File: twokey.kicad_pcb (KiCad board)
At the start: 2 copper layers, 52.1 x 40 mm, 12 parts, among them J1 12401610E4#2A, SW1 SW_SPST, SW2 SW_SPST, U1 ATSAMD21E18A-A, U2 MCP1700-3302E_SOT23

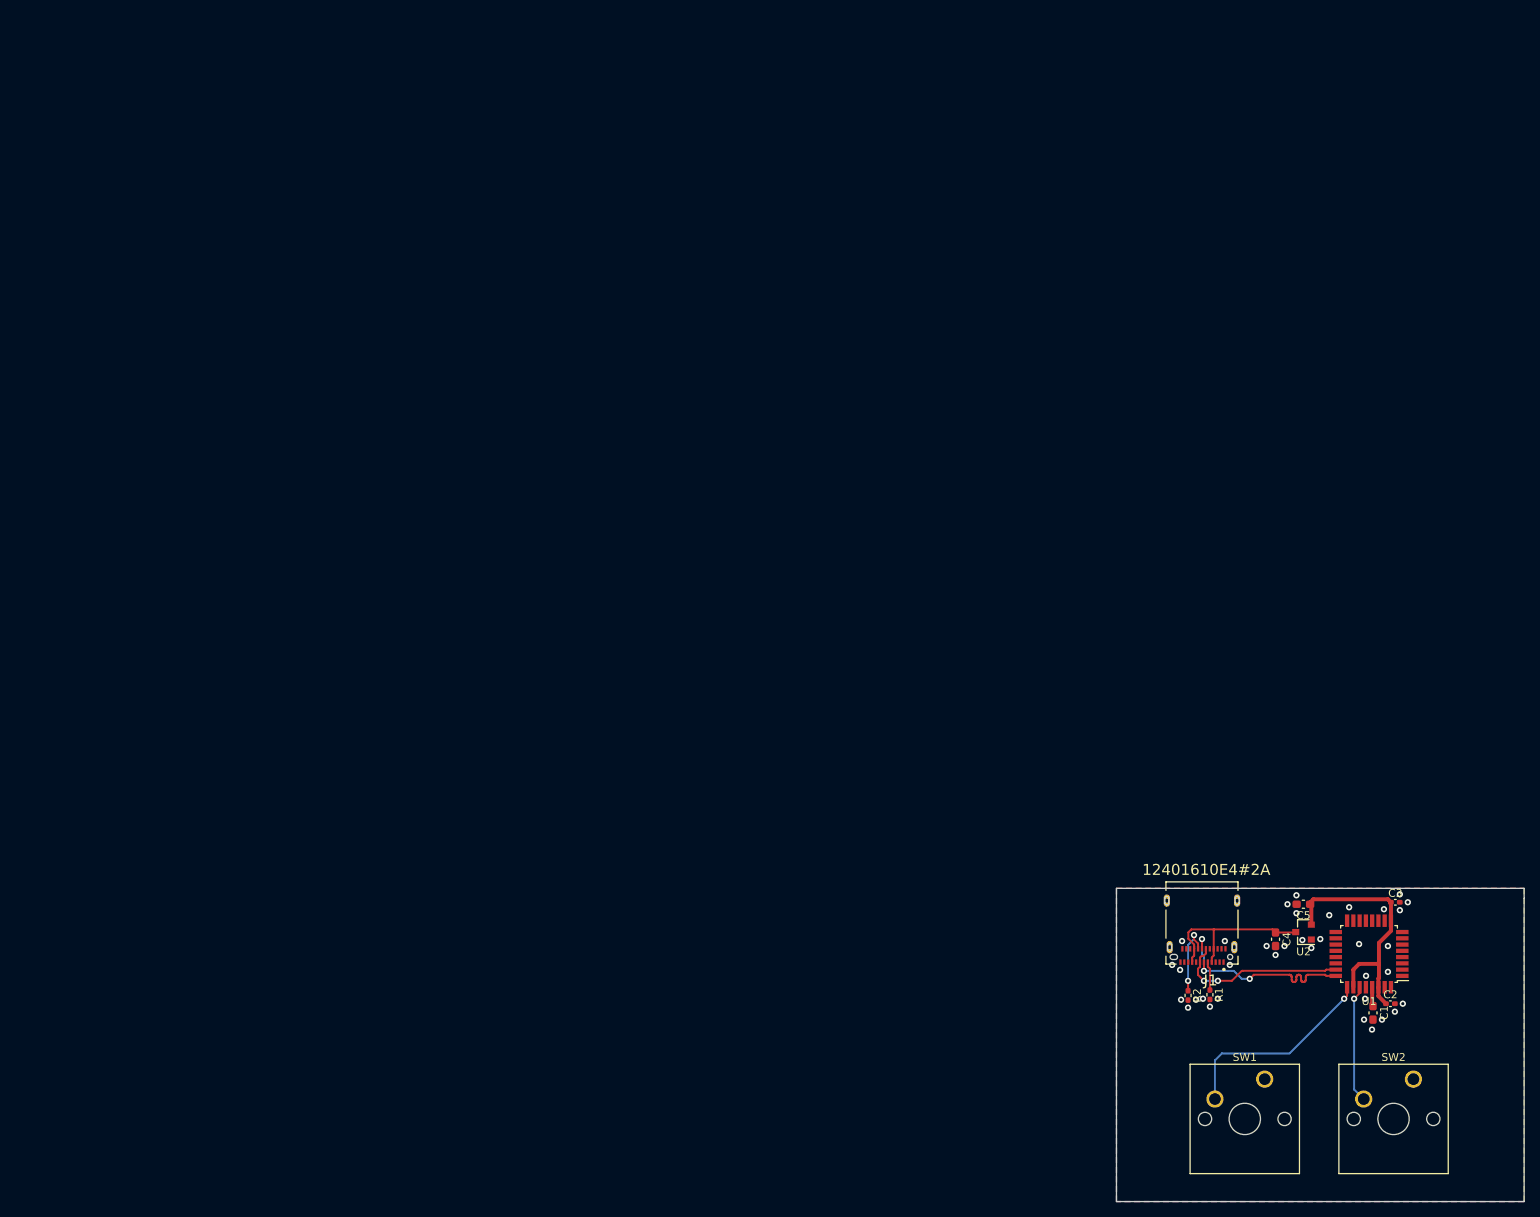
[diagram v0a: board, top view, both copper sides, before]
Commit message: ordered pcb
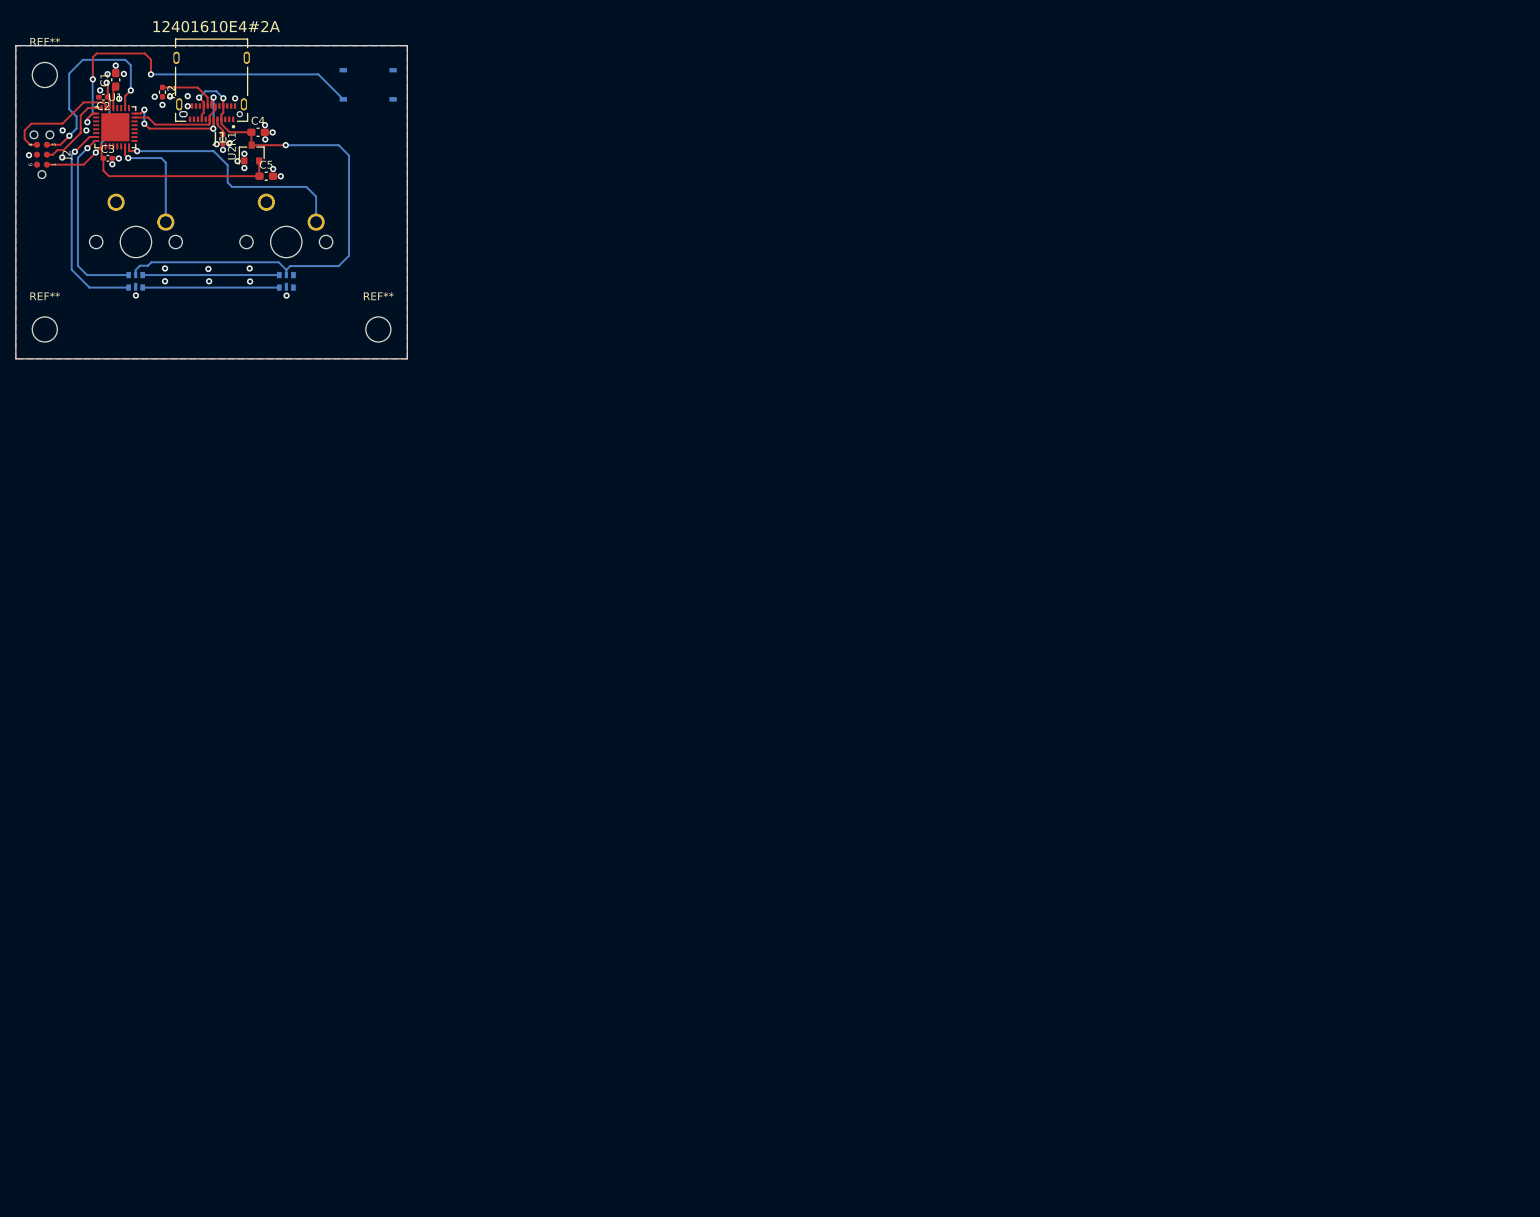
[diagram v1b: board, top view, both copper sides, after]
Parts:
- added D1: BB-2020BGR-TRB, twokey:LED_BB-2020BGR-TRB, B.Cu at (-9.70, 10.1)
- added D2: BB-2020BGR-TRB, twokey:LED_BB-2020BGR-TRB, B.Cu at (9.55, 10.1)
- added J2: Conn_02x03_Odd_Even, twokey:TC2030-IDC-NL, F.Cu at (-21.7, -6.07)
- added REF**: MountingHole_3.2mm_M3, MountingHole:MountingHole_3.2mm_M3, F.Cu at (-21.3, -16.2)
- added REF**: MountingHole_3.2mm_M3, MountingHole:MountingHole_3.2mm_M3, F.Cu at (-21.3, 16.2)
- added REF**: MountingHole_3.2mm_M3, MountingHole:MountingHole_3.2mm_M3, F.Cu at (21.3, 16.2)
- added U3: PTS526_SK15_SMTR2_LFS, twokey:PTS526 SK15 SMTR2 LFS, B.Cu at (20.0, -15.0)
- J1: footprint 12401610E4_2A:AMPHENOL_12401610E4#2A -> Digi-Key:AMPHENOL_12401610E4#2A
- SW1, SW2: moved to B.Cu
- U1: footprint Package_QFP:TQFP-32_7x7mm_P0.8mm -> Package_DFN_QFN:QFN-32-1EP_5x5mm_P0.5mm_EP3.6x3.6mm
- moved C2 201.1 mm to (-13.8, -13.4), turned to 180 degrees
- moved SW2 200.0 mm to (-12.2, 0.00), turned to 180 degrees
- moved C1 200.0 mm to (-12.2, -15.6), turned to 90 degrees
- moved U1 191.8 mm to (-12.3, -9.58), turned to 0 degrees
- moved C3 189.9 mm to (-13.3, -5.61)
- moved R2 174.5 mm to (-6.27, -14.1)
- moved SW1 169.7 mm to (7.00, 0.00), turned to 180 degrees
- moved U2 167.2 mm to (5.13, -6.28), turned to 90 degrees
- moved R1 166.9 mm to (1.45, -8.09)
- moved J1 166.1 mm to (0.00, -11.2)
- moved C4 165.9 mm to (5.94, -8.94), turned to 0 degrees
- moved C5 161.8 mm to (6.99, -3.33), turned to 0 degrees
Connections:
- U1 pad 1: Net-(U1-Pad1) -> BUTTON
- U1 pad 15: Net-(U1-Pad15) -> KEY2
- U1 pad 16: Net-(U1-Pad16) -> KEY1
- U1 pad 25: KEY1 -> Net-(U1-Pad25)
- U1 pad 26: +3V3 -> ~RESET
- U1 pad 27: KEY2 -> Net-(U1-Pad27)
- U1 pad 31: Net-(U1-Pad31) -> SWCLK
- U1 pad 32: Net-(U1-Pad32) -> SWDIO
- U1 pad 7: Net-(U1-Pad7) -> LED_DI
- U1 pad 8: Net-(U1-Pad8) -> LED_CI
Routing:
- net VBUS: track 22.6 -> 72.2 mm, vias 0 -> 3
- net BUTTON: track 0.00 -> 46.1 mm, vias 0 -> 3
- net LED_DI: track 0.00 -> 26.9 mm, vias 0 -> 1
- net ~RESET: track 0.00 -> 26.7 mm, vias 0 -> 2
- net LED_CI: track 0.00 -> 24.0 mm, vias 0 -> 1
- net Net-(D1-Pad6): track 0.00 -> 17.5 mm
- net Net-(D1-Pad1): track 0.00 -> 17.5 mm
- net SWCLK: track 0.00 -> 15.4 mm
- net +3V3: track 33.7 -> 46.5 mm, vias 0 -> 2
- net SWDIO: track 0.00 -> 10.8 mm
- net D-: track 22.4 -> 12.6 mm, vias 2 -> 0
- net D+: track 26.8 -> 19.4 mm, vias 3 -> 4
- net KEY1: track 26.3 -> 31.4 mm
- net Net-(J1-PadB5): track 9.65 -> 7.39 mm, vias 2 -> 0
- net Net-(J1-PadA5): track 3.68 -> 2.19 mm
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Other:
- board size 52.1 x 40 mm -> 50 x 40 mm
- net class +3.3V: trace_width 0.508 -> 0.25
- net class VBUS added: clearance 0.2, trace_width 0.25, via_dia 0.8, via_drill 0.4
